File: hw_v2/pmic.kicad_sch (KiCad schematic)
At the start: 17 parts, among them U2 TC4424A, U3 TC4424A

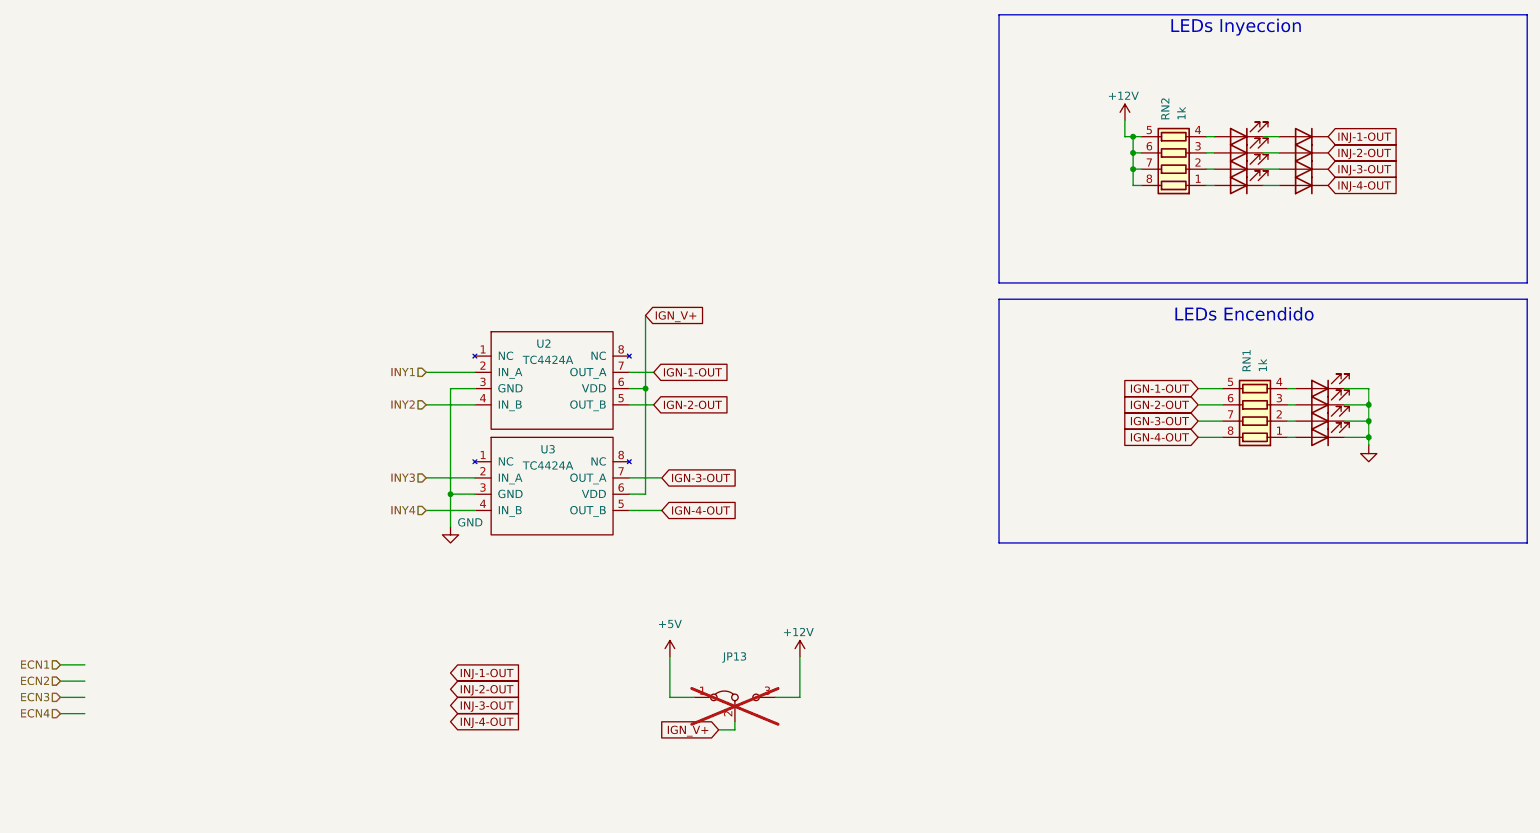
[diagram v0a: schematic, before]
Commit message: WIP v7
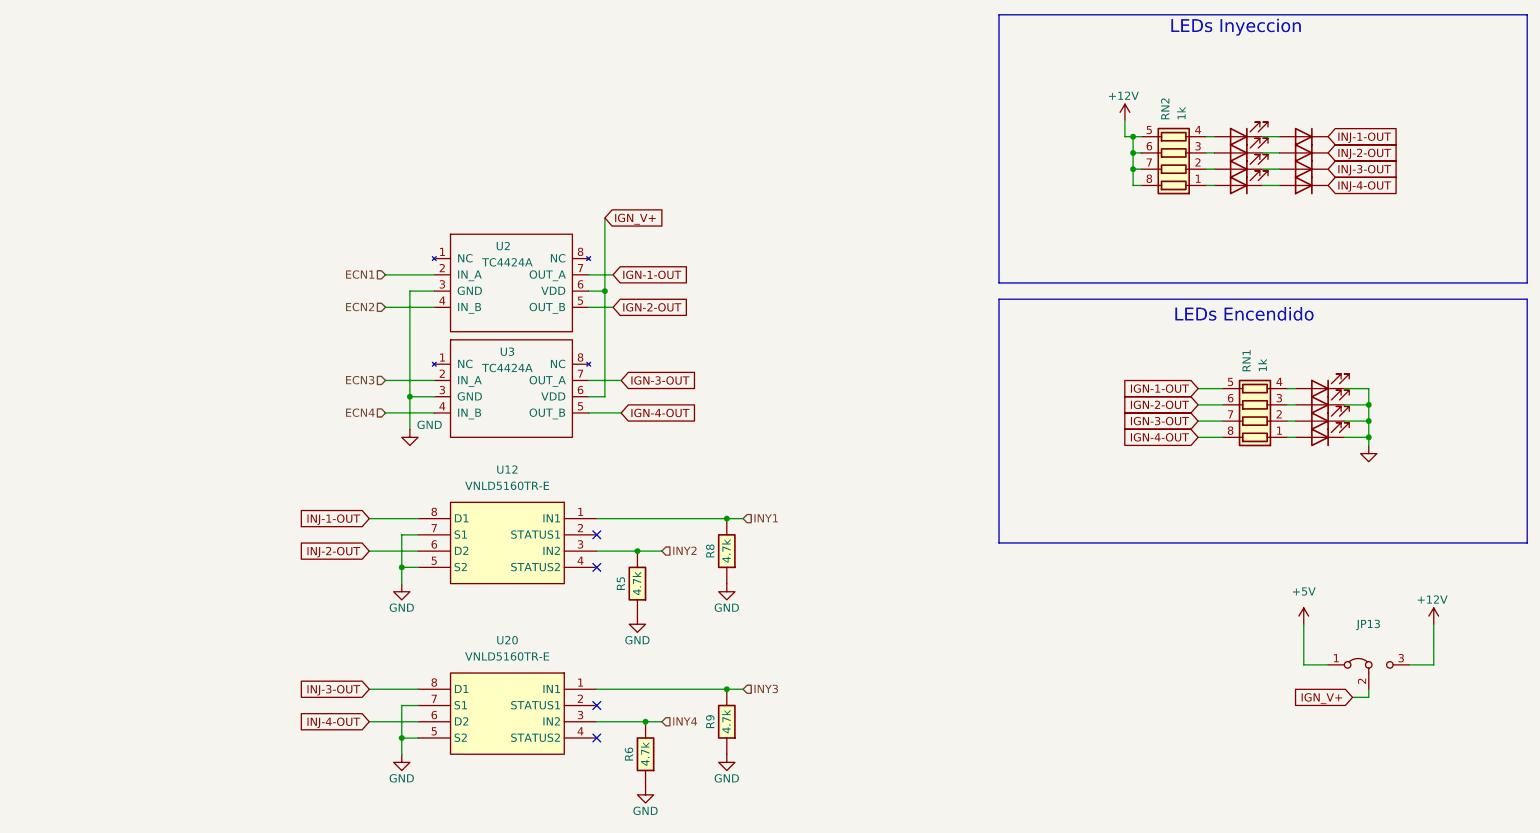
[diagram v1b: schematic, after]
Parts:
- added R5, R6, R8, R9: 4.7k, hellen-one-common:R0603, symbol hellen-one-common:Res
- added U12, U20: VNLD5160TR-E, Package_SO:SOIC-8_3.9x4.9mm_P1.27mm, symbol chips:VNLD5160
- JP13: now fitted
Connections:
- net ECN1: now also U2.2 (IN_A)
- net ECN2: now also U2.4 (IN_B)
- net ECN3: now also U3.2 (IN_A)
- net ECN4: now also U3.4 (IN_B)
- net GND: now also R5.1, R6.1, R8.1, R9.1, U12.5 (S2), U12.7 (S1), U20.5 (S2), U20.7 (S1)
- net INJ-1-OUT: now also U12.8 (D1)
- net INJ-2-OUT: now also U12.6 (D2)
- net INJ-3-OUT: now also U20.8 (D1)
- net INJ-4-OUT: now also U20.6 (D2)
- net INY1: now also R8.2, U12.1 (IN1); no longer U2.2 (IN_A)
- net INY2: now also R5.2, U12.3 (IN2); no longer U2.4 (IN_B)
- net INY3: now also R9.2, U20.1 (IN1); no longer U3.2 (IN_A)
- net INY4: now also R6.2, U20.3 (IN2); no longer U3.4 (IN_B)
- no-connect marks 0 -> 4
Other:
- moved on the sheet: U2, U3

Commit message: hw v2
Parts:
- R5, R6, R8, R9: footprint hellen-one-common:R0603 -> Resistor_SMD:R_0603_1608Metric
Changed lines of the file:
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@@
 			)
 		)
-		(property "Footprint" "hellen-one-common:R0603"
+		(property "Footprint" "Resistor_SMD:R_0603_1608Metric"
 			(at 142.24 135.89 0)
 			(effects
@@
 			)
 		)
-		(property "Footprint" "hellen-one-common:R0603"
+		(property "Footprint" "Resistor_SMD:R_0603_1608Metric"
 			(at 154.94 104.14 0)
 			(effects
@@
 			)
 		)
-		(property "Footprint" "hellen-one-common:R0603"
+		(property "Footprint" "Resistor_SMD:R_0603_1608Metric"
 			(at 154.94 130.81 0)
 			(effects
@@
 			)
 		)
-		(property "Footprint" "hellen-one-common:R0603"
+		(property "Footprint" "Resistor_SMD:R_0603_1608Metric"
 			(at 140.97 109.22 0)
 			(effects
